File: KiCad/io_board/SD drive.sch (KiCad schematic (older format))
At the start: 29 parts, among them J3 SD_Card, J4 JTAG, U12 AMS1117-3.3, U13 SN74LVC245A, U14 74HCT32, U15 SN74LVC8T245PWR, U7 EPM240T100, X2 10 MHz

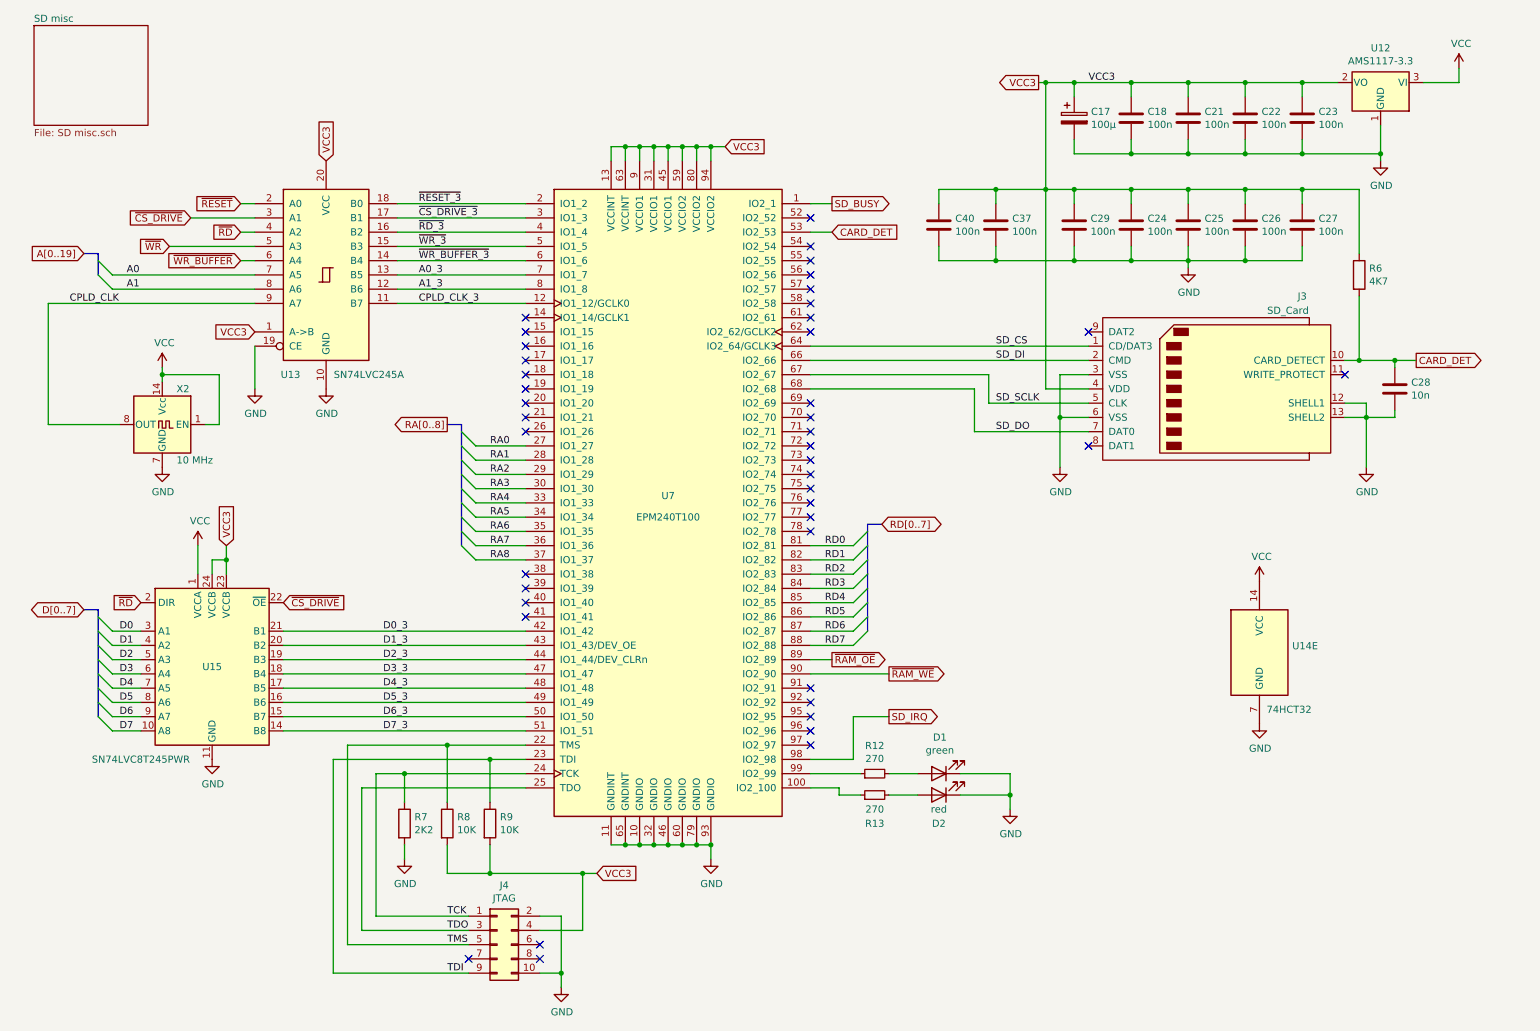
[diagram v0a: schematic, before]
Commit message: Updated I/O board
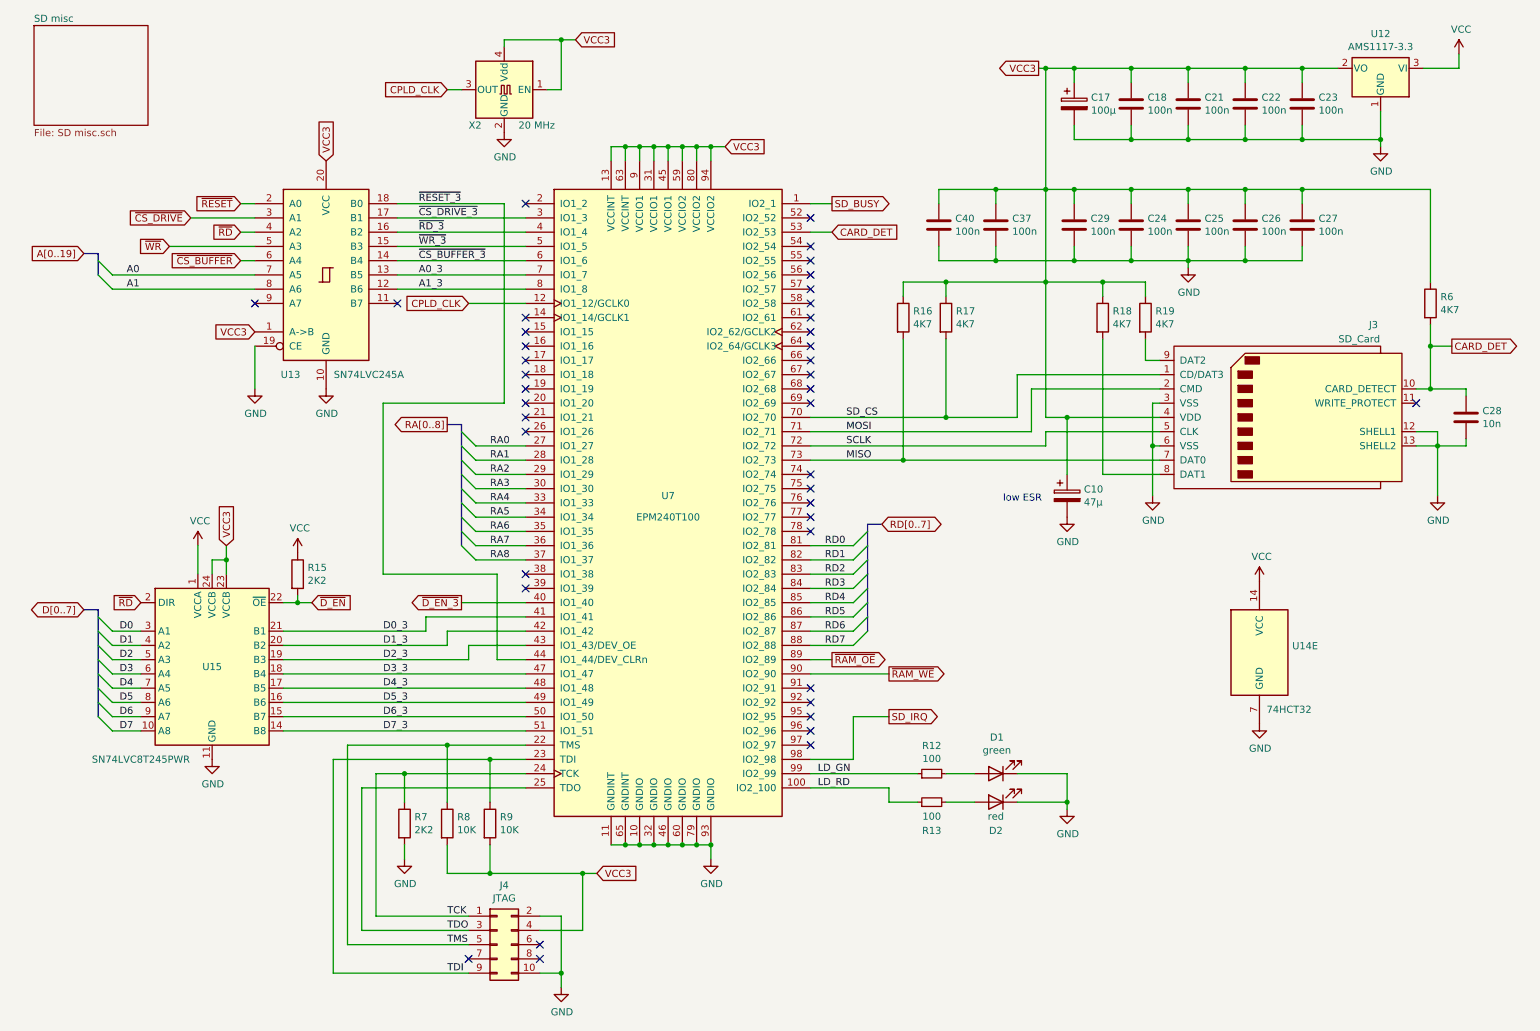
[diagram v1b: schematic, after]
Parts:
- removed X2: 10 MHz, Oscillator:Oscillator_DIP-14, symbol Oscillator:CXO_DIP14
- added C10: 47µ, Capacitor_SMD:CP_Elec_5x5.4, symbol Device:CP
- added R15: 2K2, Resistor_SMD:R_1206_3216Metric, symbol Device:R
- added R16, R17, R18, R19: 4K7, Resistor_SMD:R_1206_3216Metric, symbol Device:R
- added X2: 20 MHz, Oscillator:Oscillator_SMD_Abracon_ASV-4Pin_7.0x5.1mm, symbol Oscillator:ASV-xxxMHz
- C17: footprint Capacitor_THT:CP_Radial_D5.0mm_P2.50mm -> Capacitor_SMD:CP_Elec_5x5.4
- R12, R13: value 270 -> 100
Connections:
- net CPLD_CLK: now also U7.12 (IO1_12/GCLK0), X2.3 (OUT); no longer U13.9 (A7)
- net D0_3: now also U7.41 (IO1_41); no longer U7.42 (IO1_42)
- net D1_3: now also U7.42 (IO1_42); no longer U7.43 (IO1_43/DEV_OE)
- net D2_3: now also U7.43 (IO1_43/DEV_OE); no longer U7.44 (IO1_44/DEV_CLRn)
- net GND: now also C10.2, X2.2 (GND)
- net SD_CS: now also U7.70 (IO2_70), R17.2; no longer U7.64 (IO2_64/GCLK3)
- net VCC: now also R15.1
- net VCC3: now also C10.1, R16.1, R17.1, R18.1, R19.1, X2.1 (EN), X2.4 (Vdd)
- net ~CS_DRIVE: no longer U15.22 (~OE)
- net ~RESET_3: now also U7.44 (IO1_44/DEV_CLRn); no longer U7.2 (IO1_2)
- net at J3.8 (DAT1): now also R18.2
- net at J3.9 (DAT2): now also R19.2
- net LD_RD: now reaches R13.1, U7.100 (IO2_100)
- net ~D_EN_3: now reaches U7.40 (IO1_40)
- net MOSI: now reaches U7.71 (IO2_71)
- net MOSI: now also J3.2 (CMD)
- net SCLK: now reaches U7.72 (IO2_72)
- net SCLK: now also J3.5 (CLK)
- net MISO: now reaches U7.73 (IO2_73)
- net MISO: now also J3.7 (DAT0), R16.2
- net LD_GN: now reaches R12.1, U7.99 (IO2_99)
- net CPLD_CLK_3: no longer names the net of U13.11 (B7)
- net CPLD_CLK_3: no longer U7.12 (IO1_12/GCLK0)
- net SD_DI: no longer names the net of U7.66 (IO2_66)
- net SD_DI: no longer J3.2 (CMD)
- net SD_DO: no longer names the net of U7.68 (IO2_68)
- net SD_DO: no longer J3.7 (DAT0)
- net SD_SCLK: no longer names the net of U7.67 (IO2_67)
- net SD_SCLK: no longer J3.5 (CLK)
- net ~WR_BUFFER renamed ~CS_BUFFER
- net ~WR_BUFFER_3 renamed ~CS_BUFFER_3
- new net ~D_EN: R15.2, U15.22 (~OE)
- no-connect marks 42 -> 41
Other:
- note added: "low ESR"
- moved on the sheet: C17, C18, C21, C22, C23, C28, D1, D2, J3, R12, R13, R6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
